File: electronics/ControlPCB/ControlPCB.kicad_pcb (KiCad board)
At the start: 2 copper layers, 70 parts, among them CON1 12VINPUT, P1 CONN_02X03, P2 CONN_02X03, P3 CONN_02X03, P4 CONN_02X03, P5 CONN_02X03, P6 CONN_02X03, P7 CONN_02X03, P8 CONN_02X03, U1 POLOLU_A4988, U2 POLOLU_A4988, U3 POLOLU_A4988, U4 POLOLU_A4988, U5 POLOLU_A4988, U6 POLOLU_A4988, U7 POLOLU_A4988, U8 POLOLU_A4988

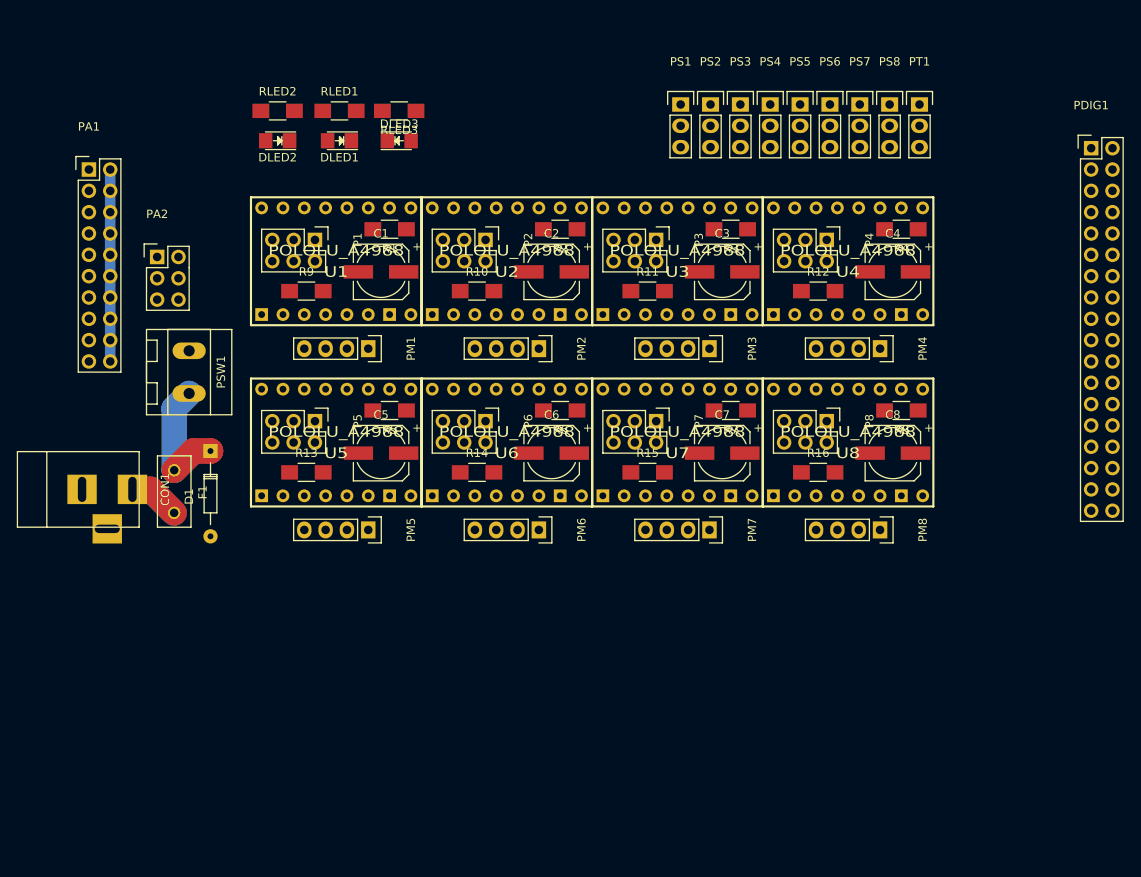
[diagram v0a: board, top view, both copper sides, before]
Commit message: ControlPCB before square
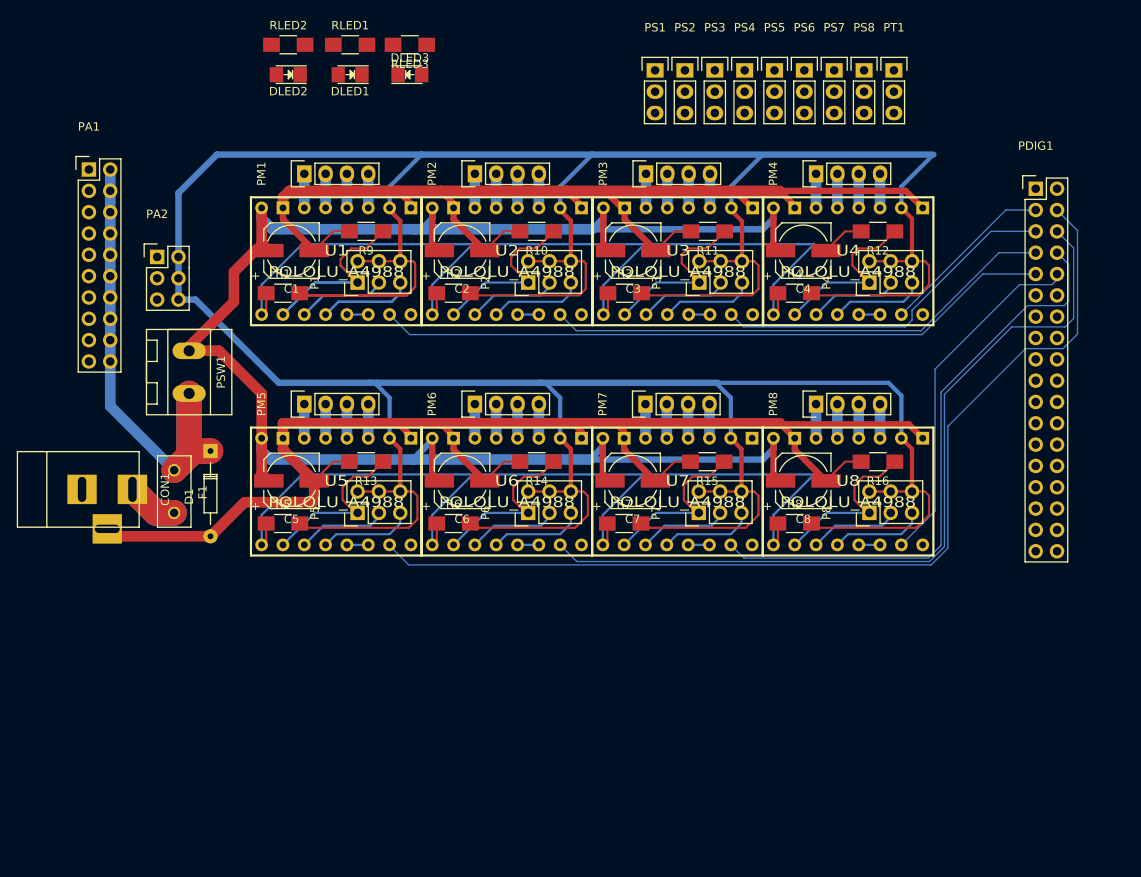
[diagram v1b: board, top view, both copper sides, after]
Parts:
- moved PM1 22.2 mm to (96.5, 58.2), turned to 90 degrees
- moved PM4 22.2 mm to (157.5, 58.2), turned to 90 degrees
- moved PM2 22.2 mm to (116.8, 58.2), turned to 90 degrees
- moved PM3 22.2 mm to (137.2, 58.2), turned to 90 degrees
- moved R5 18.5 mm to (94.0, 99.8), turned to 0 degrees
- moved R6 18.5 mm to (114.3, 99.8), turned to 0 degrees
- moved R7 18.5 mm to (134.6, 99.8), turned to 0 degrees
- moved R8 18.5 mm to (154.9, 99.8), turned to 0 degrees
- moved PM5 16.8 mm to (96.5, 85.6), turned to 90 degrees
- moved PM7 16.8 mm to (137.2, 85.6), turned to 90 degrees
- moved PM8 16.8 mm to (157.5, 85.6), turned to 90 degrees
- moved PM6 16.8 mm to (116.8, 85.6), turned to 90 degrees
- moved R1 14.8 mm to (94.0, 72.4), turned to 0 degrees
- moved R2 14.8 mm to (114.3, 72.4), turned to 0 degrees
- moved R4 14.8 mm to (154.9, 72.4), turned to 0 degrees
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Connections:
- P1 pad 1: VCC -> Net-(P1-Pad1)
- P1 pad 2: Net-(P1-Pad2) -> VCC
- P1 pad 3: VCC -> Net-(P1-Pad3)
- P1 pad 4: Net-(P1-Pad4) -> VCC
- P1 pad 5: VCC -> Net-(P1-Pad5)
- P1 pad 6: Net-(P1-Pad6) -> VCC
- P2 pad 1: VCC -> Net-(P2-Pad1)
- P2 pad 2: Net-(P2-Pad2) -> VCC
- P2 pad 3: VCC -> Net-(P2-Pad3)
- P2 pad 4: Net-(P2-Pad4) -> VCC
- P2 pad 5: VCC -> Net-(P2-Pad5)
- P2 pad 6: Net-(P2-Pad6) -> VCC
- P3 pad 1: VCC -> Net-(P3-Pad1)
- P3 pad 2: Net-(P3-Pad2) -> VCC
- P3 pad 3: VCC -> Net-(P3-Pad3)
- P3 pad 4: Net-(P3-Pad4) -> VCC
- P3 pad 5: VCC -> Net-(P3-Pad5)
- P3 pad 6: Net-(P3-Pad6) -> VCC
- P4 pad 1: VCC -> Net-(P4-Pad1)
- P4 pad 2: Net-(P4-Pad2) -> VCC
- P4 pad 3: VCC -> Net-(P4-Pad3)
- P4 pad 4: Net-(P4-Pad4) -> VCC
- P4 pad 5: VCC -> Net-(P4-Pad5)
- P4 pad 6: Net-(P4-Pad6) -> VCC
- P5 pad 1: VCC -> Net-(P5-Pad1)
- P5 pad 2: Net-(P5-Pad2) -> VCC
- P5 pad 3: VCC -> Net-(P5-Pad3)
- P5 pad 4: Net-(P5-Pad4) -> VCC
- P5 pad 5: VCC -> Net-(P5-Pad5)
- P5 pad 6: Net-(P5-Pad6) -> VCC
- P6 pad 1: VCC -> Net-(P6-Pad1)
- P6 pad 2: Net-(P6-Pad2) -> VCC
- P6 pad 3: VCC -> Net-(P6-Pad3)
- P6 pad 4: Net-(P6-Pad4) -> VCC
- P6 pad 5: VCC -> Net-(P6-Pad5)
- P6 pad 6: Net-(P6-Pad6) -> VCC
- P7 pad 1: VCC -> Net-(P7-Pad1)
- P7 pad 2: Net-(P7-Pad2) -> VCC
- P7 pad 3: VCC -> Net-(P7-Pad3)
- P7 pad 4: Net-(P7-Pad4) -> VCC
- P7 pad 5: VCC -> Net-(P7-Pad5)
- P7 pad 6: Net-(P7-Pad6) -> VCC
- P8 pad 1: VCC -> Net-(P8-Pad1)
- P8 pad 2: Net-(P8-Pad2) -> VCC
- P8 pad 3: VCC -> Net-(P8-Pad3)
- P8 pad 4: Net-(P8-Pad4) -> VCC
- P8 pad 5: VCC -> Net-(P8-Pad5)
- P8 pad 6: Net-(P8-Pad6) -> VCC
- PDIG1 pad 3: STEPM1 -> STEPM4
- PDIG1 pad 4: STEPM2 -> STEPM5
- PDIG1 pad 6: STEPM4 -> STEPM6
- PDIG1 pad 7: STEPM5 -> STEPM2
- PDIG1 pad 8: STEPM6 -> STEPM7
- PDIG1 pad 9: STEPM7 -> STEPM1
- R10 pad 1: Net-(P2-Pad2) -> Net-(P2-Pad5)
- R11 pad 1: Net-(P3-Pad2) -> Net-(P3-Pad5)
- R12 pad 1: Net-(P4-Pad2) -> Net-(P4-Pad5)
- R13 pad 1: Net-(P5-Pad2) -> Net-(P5-Pad5)
- R14 pad 1: Net-(P6-Pad2) -> Net-(P6-Pad5)
- R15 pad 1: Net-(P7-Pad2) -> Net-(P7-Pad5)
- R16 pad 1: Net-(P8-Pad2) -> Net-(P8-Pad5)
- R9 pad 1: Net-(P1-Pad2) -> Net-(P1-Pad5)
- U1 pad 10: Net-(P1-Pad2) -> Net-(P1-Pad5)
- U1 pad 11: Net-(P1-Pad4) -> Net-(P1-Pad3)
- U1 pad 12: Net-(P1-Pad6) -> Net-(P1-Pad1)
- U2 pad 10: Net-(P2-Pad2) -> Net-(P2-Pad5)
- U2 pad 11: Net-(P2-Pad4) -> Net-(P2-Pad3)
- U2 pad 12: Net-(P2-Pad6) -> Net-(P2-Pad1)
- U3 pad 10: Net-(P3-Pad2) -> Net-(P3-Pad5)
- U3 pad 11: Net-(P3-Pad4) -> Net-(P3-Pad3)
- U3 pad 12: Net-(P3-Pad6) -> Net-(P3-Pad1)
- U4 pad 10: Net-(P4-Pad2) -> Net-(P4-Pad5)
- U4 pad 11: Net-(P4-Pad4) -> Net-(P4-Pad3)
- U4 pad 12: Net-(P4-Pad6) -> Net-(P4-Pad1)
- U5 pad 10: Net-(P5-Pad2) -> Net-(P5-Pad5)
- U5 pad 11: Net-(P5-Pad4) -> Net-(P5-Pad3)
- U5 pad 12: Net-(P5-Pad6) -> Net-(P5-Pad1)
- U6 pad 10: Net-(P6-Pad2) -> Net-(P6-Pad5)
- U6 pad 11: Net-(P6-Pad4) -> Net-(P6-Pad3)
- U6 pad 12: Net-(P6-Pad6) -> Net-(P6-Pad1)
- U7 pad 10: Net-(P7-Pad2) -> Net-(P7-Pad5)
- U7 pad 11: Net-(P7-Pad4) -> Net-(P7-Pad3)
- U7 pad 12: Net-(P7-Pad6) -> Net-(P7-Pad1)
- U8 pad 10: Net-(P8-Pad2) -> Net-(P8-Pad5)
- U8 pad 11: Net-(P8-Pad4) -> Net-(P8-Pad3)
- U8 pad 12: Net-(P8-Pad6) -> Net-(P8-Pad1)
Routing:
- net VCC: track 0.00 -> 523.0 mm
- net GND: track 0.00 -> 303.0 mm
- net ENABLEM: track 0.00 -> 227.2 mm
- net +12V: track 0.00 -> 219.6 mm
- net STEPM5: track 0.00 -> 118.7 mm
- net STEPM6: track 0.00 -> 95.8 mm
- net STEPM1: track 0.00 -> 80.9 mm
- net STEPM7: track 0.00 -> 70.6 mm
- net STEPM2: track 0.00 -> 61.3 mm
- net STEPM3: track 0.00 -> 42.3 mm
- net STEPM8: track 0.00 -> 42.3 mm
- net Net-(P1-Pad5): track 0.00 -> 34.6 mm
- net Net-(P1-Pad1): track 0.00 -> 22.4 mm
- net VDD: track 43.8 -> 65.2 mm
- net Net-(P1-Pad3): track 0.00 -> 21.2 mm
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
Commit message: ControlPCB update
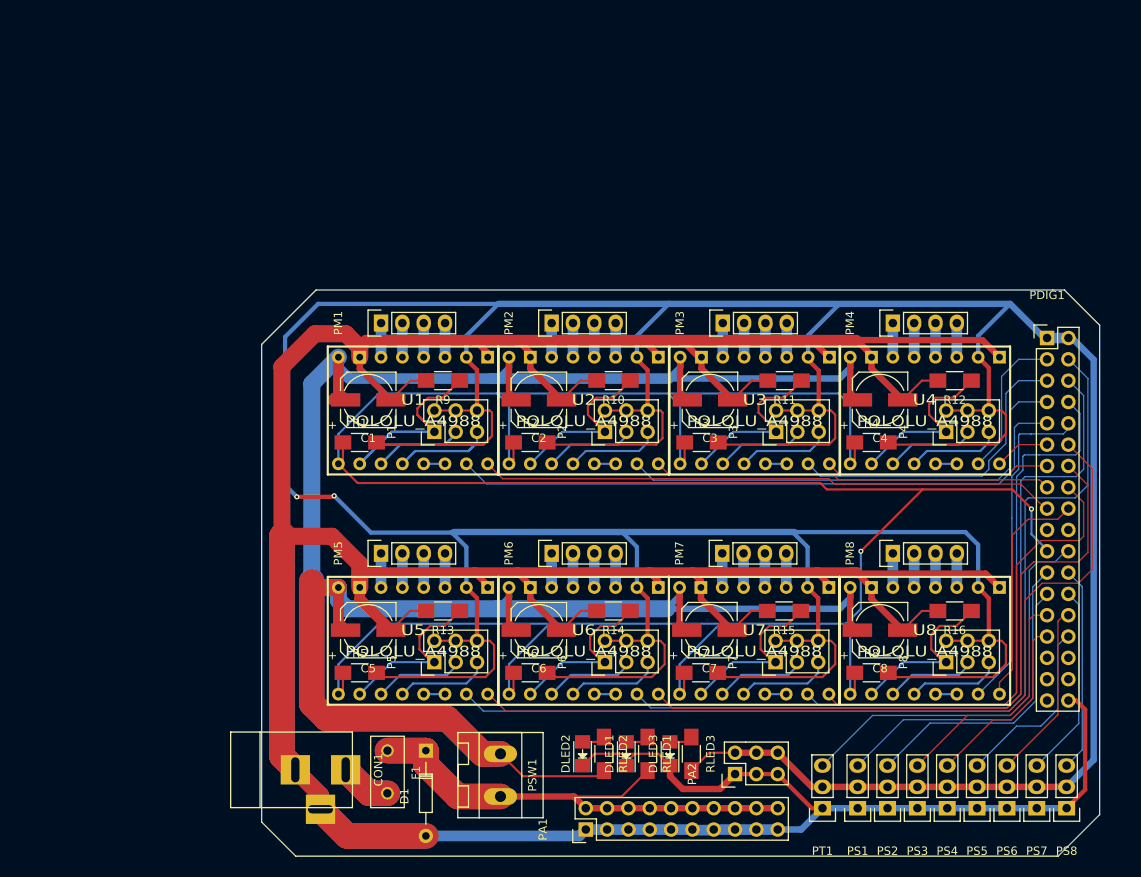
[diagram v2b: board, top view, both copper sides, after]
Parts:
- moved PA1 98.4 mm to (130.0, 136.3), turned to 90 degrees
- moved RLED2 92.4 mm to (132.2, 127.3), turned to 270 degrees
- moved PA2 92.4 mm to (147.8, 129.7), turned to 90 degrees
- moved RLED1 91.6 mm to (137.4, 127.3), turned to 270 degrees
- moved PS1 91.1 mm to (162.4, 133.7), turned to 180 degrees
- moved PS2 91.1 mm to (166.0, 133.7), turned to 180 degrees
- moved PS3 91.1 mm to (169.5, 133.7), turned to 180 degrees
- moved PS4 91.1 mm to (173.1, 133.7), turned to 180 degrees
- moved PS5 91.1 mm to (176.7, 133.7), turned to 180 degrees
- moved PS6 91.1 mm to (180.2, 133.7), turned to 180 degrees
- moved PS7 91.1 mm to (183.8, 133.7), turned to 180 degrees
- moved PS8 91.1 mm to (187.3, 133.7), turned to 180 degrees
- moved RLED3 90.9 mm to (142.6, 127.3), turned to 270 degrees
- moved PT1 88.3 mm to (158.2, 133.7), turned to 180 degrees
- moved DLED2 88.2 mm to (129.7, 127.3), turned to 90 degrees
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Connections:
- PDIG1 pad 11: DIRM1 -> DIRM4
- PDIG1 pad 12: DIRM2 -> DIRM5
- PDIG1 pad 14: DIRM4 -> DIRM6
- PDIG1 pad 15: DIRM5 -> DIRM2
- PDIG1 pad 16: DIRM6 -> DIRM7
- PDIG1 pad 17: DIRM7 -> DIRM1
- PDIG1 pad 24: SOPTO2 -> SOPTO8
- PDIG1 pad 25: SOPTO3 -> SOPTO2
- PDIG1 pad 26: SOPTO4 -> SOPTO7
- PDIG1 pad 27: SOPTO5 -> SOPTO3
- PDIG1 pad 29: SOPTO7 -> SOPTO4
- PDIG1 pad 30: SOPTO8 -> SOPTO5
- PDIG1 pad 35: GND -> Net-(PDIG1-Pad35)
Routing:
- net GND: track 303.0 -> 550.2 mm
- net VCC: track 523.0 -> 631.9 mm, vias 0 -> 2
- net DIRM5: track 0.00 -> 102.5 mm
- net +12V: track 219.6 -> 319.4 mm
- net ENABLEM: track 227.2 -> 320.2 mm, vias 0 -> 2
- net DIRM6: track 0.00 -> 79.2 mm
- net DIRM1: track 0.00 -> 68.8 mm
- net DIRM7: track 0.00 -> 54.9 mm
- net STOOL: track 0.00 -> 48.6 mm
- net DIRM2: track 0.00 -> 47.5 mm
- net SOPTO1: track 0.00 -> 40.4 mm
- net SOPTO2: track 0.00 -> 34.2 mm
- net SOPTO3: track 0.00 -> 28.2 mm
- net DIRM8: track 0.00 -> 27.6 mm
- net DIRM3: track 0.00 -> 26.9 mm
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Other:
- board outline added: 99.8 x 67.4 mm
- net class Default: clearance 0 -> 0.0762
- rule trace_clearance: 0 -> 0.0762
- rule via_min_size: 0.6096 -> 0.3048
